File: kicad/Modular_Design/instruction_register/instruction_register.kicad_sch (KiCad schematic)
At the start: 7 parts

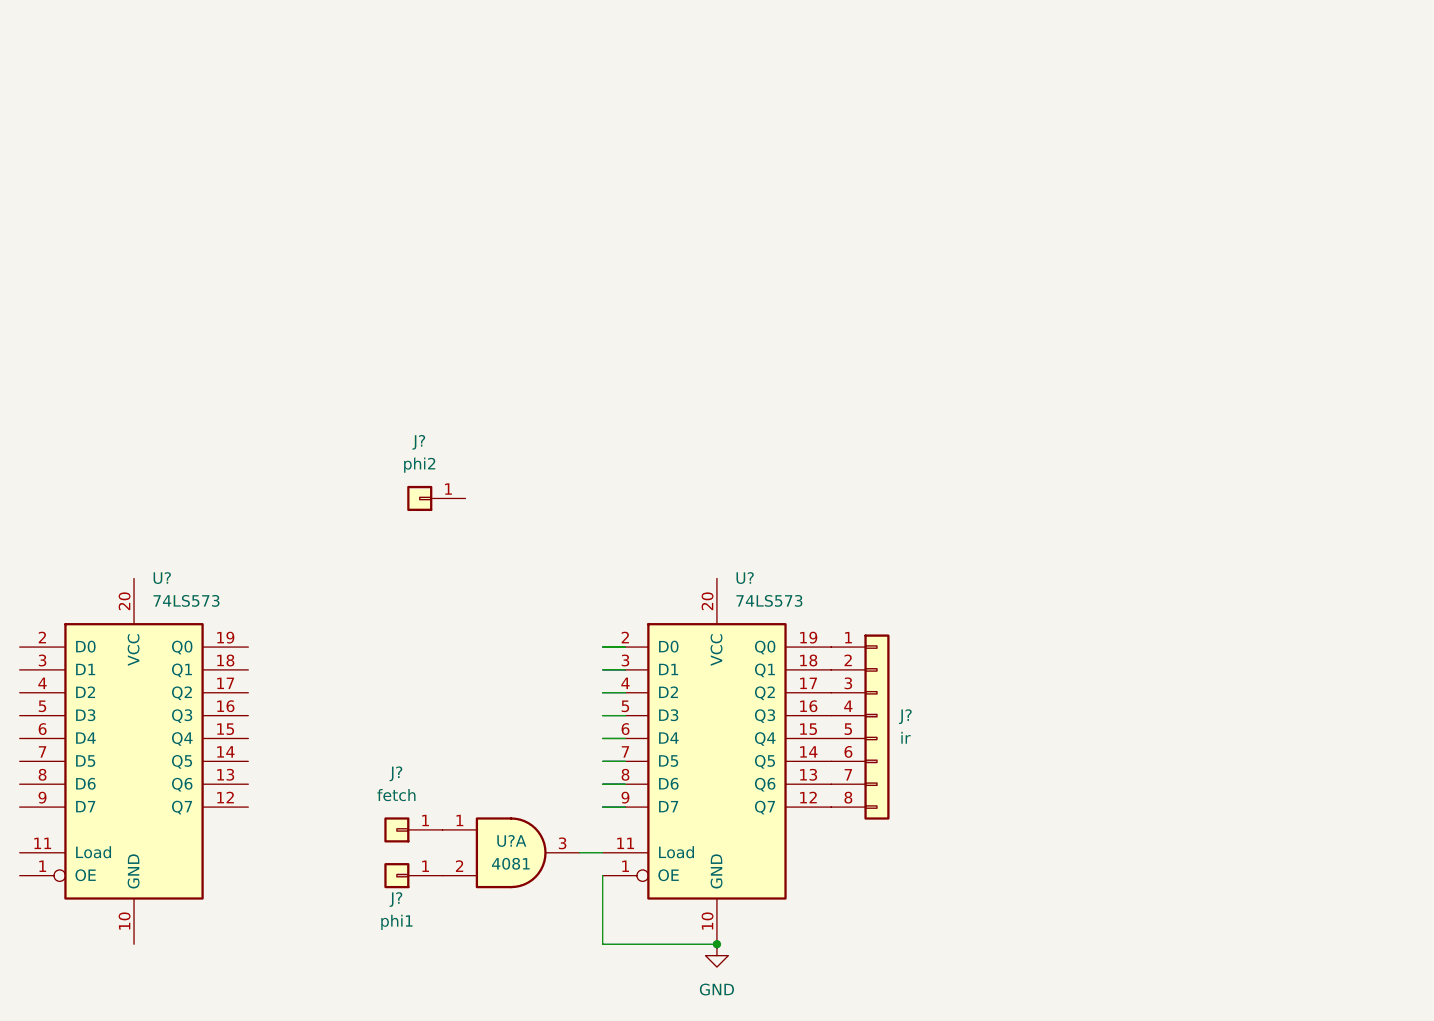
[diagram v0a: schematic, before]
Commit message: PD 70% impl
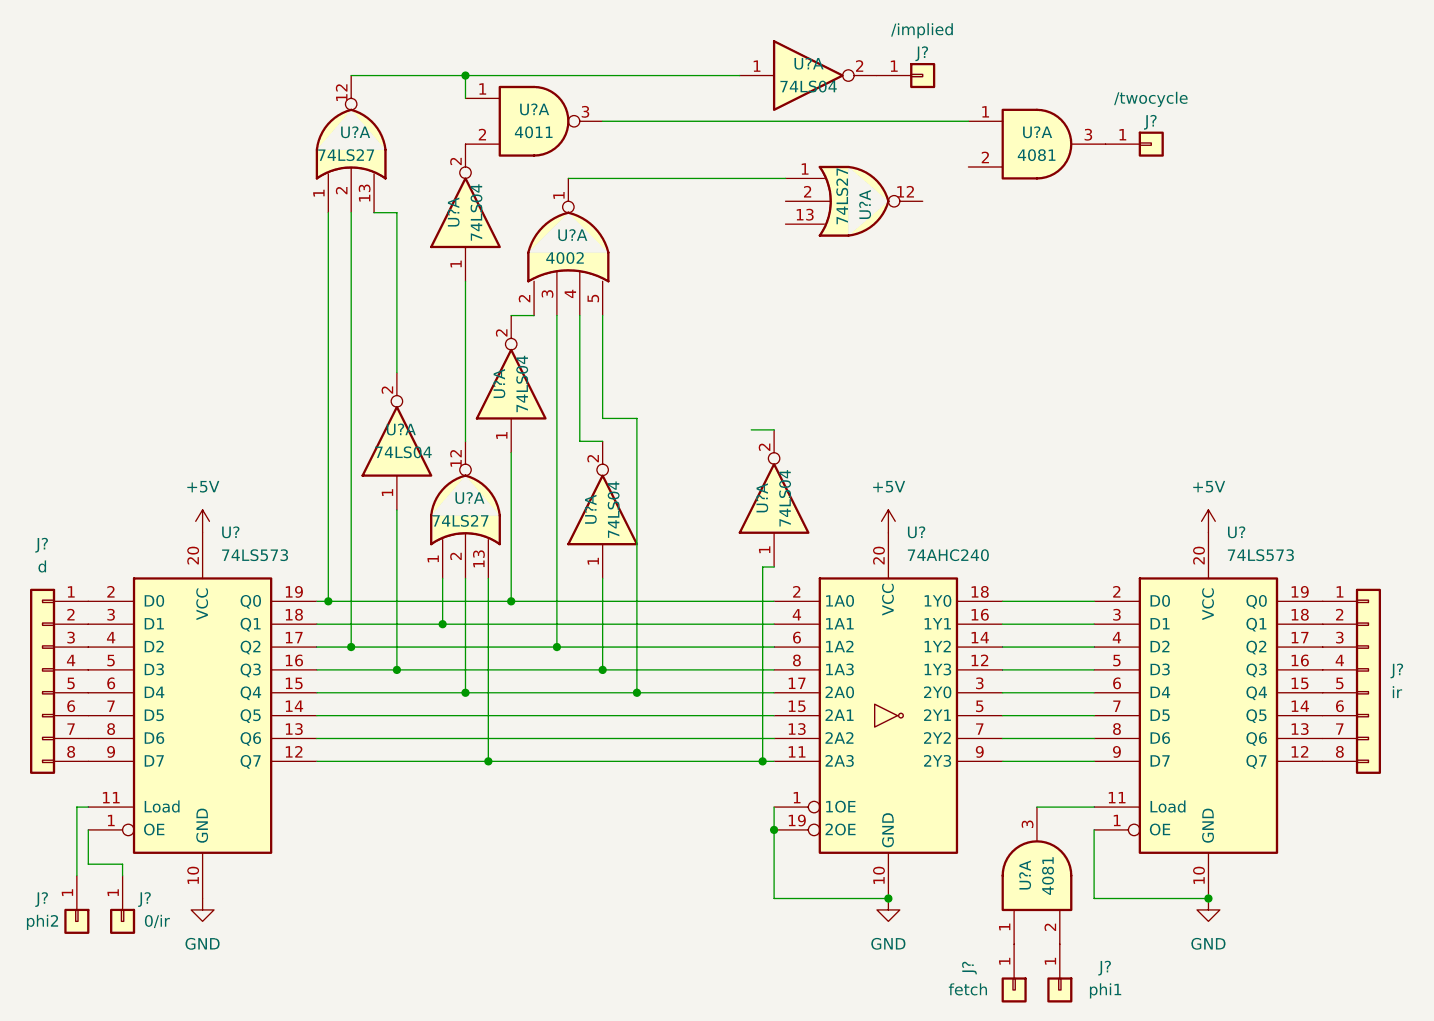
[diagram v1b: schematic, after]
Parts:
- added J?: /implied, symbol Connector_Generic:Conn_01x01
- added J?: d, symbol Connector_Generic:Conn_01x08
- added J?: 0/ir, symbol Connector_Generic:Conn_01x01
- added J?: /twocycle, symbol Connector_Generic:Conn_01x01
- added U?: 4002, symbol 4xxx:4002
- added U? (x3): 74LS27, symbol 74xx:74LS27
- added U? (x6): 74LS04, symbol 74xx:74LS04
- added U?: 74AHC240, symbol 74xx:74AHC240
- added U?: 4081, symbol 4xxx:4081
- added U?: 4011, symbol 4xxx:4011
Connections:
- net GND: now also U?.10 (GND), U?.1 (1OE), U?.10 (GND), U?.19 (2OE)
- net at U?.1 (OE): now also J?.1 (Pin_1)
- net at U?.11 (Load): now also J?.1 (Pin_1)
- net at U?.12 (Q7): now also U?.1, U?.11 (2A3), U?.13
- net at U?.13 (Q6): now also U?.13 (2A2)
- net at U?.14 (Q5): now also U?.15 (2A1)
- net at U?.15 (Q4): now also U?.17 (2A0), U?.2, U?.5
- net at U?.16 (Q3): now also U?.1, U?.1, U?.8 (1A3)
- net at U?.17 (Q2): now also U?.2, U?.3, U?.6 (1A2)
- net at U?.18 (Q1): now also U?.1, U?.4 (1A1)
- net at U?.19 (Q0): now also U?.1, U?.1, U?.2 (1A0)
- net at U?.2 (D0): now also J?.1 (Pin_1)
- net +5V: now reaches U?.20 (VCC)
- net +5V: now also U?.20 (VCC), U?.20 (VCC)
- net at U?.3 (D1): now also J?.2 (Pin_2)
- net at U?.4 (D2): now also J?.3 (Pin_3)
- net at U?.5 (D3): now also J?.4 (Pin_4)
- net at U?.6 (D4): now also J?.5 (Pin_5)
- net at U?.7 (D5): now also J?.6 (Pin_6)
- net at U?.8 (D6): now also J?.7 (Pin_7)
- net at U?.9 (D7): now also J?.8 (Pin_8)
- net at U?.2 (D0): now also U?.18 (1Y0)
- net at U?.3 (D1): now also U?.16 (1Y1)
- net at U?.4 (D2): now also U?.14 (1Y2)
- net at U?.5 (D3): now also U?.12 (1Y3)
- net at U?.6 (D4): now also U?.3 (2Y0)
- net at U?.7 (D5): now also U?.5 (2Y1)
- net at U?.8 (D6): now also U?.7 (2Y2)
- net at U?.9 (D7): now also U?.9 (2Y3)
- new net: U?.1, U?.1
- new net: U?.2, U?.2 (x2)
- new net: U?.2, U?.4
- new net: J?.1 (Pin_1), U?.2
- new net: U?.1, U?.12
- new net: U?.1, U?.1, U?.12
- new net: U?.13, U?.2
- new net: U?.1, U?.3
- new net: J?.1 (Pin_1), U?.3
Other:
- moved on the sheet: J?, U?, U?A
